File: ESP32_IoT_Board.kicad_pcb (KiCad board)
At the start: 4 copper layers, 127.9 x 63.9 mm, 98 parts, among them J1 SS-52400-002, J2 B2B-PH-SM4-TB, J3 GSD090012SEU, J4 Conn_01x04_Pin, Q1 TEMT6000X01, Q2 BC817, Q3 BC817, U1 MCP73871-2CAI_ML, U2 BME280, U3 ESP32-C3-WROOM-02-H4, U4 CP2102N-Axx-xQFN20, U5 USBLC6-2SC6, U6 W25Q32JVSSIQ, U7 MAX4466EXK, U8 LM1117MPX-3.3

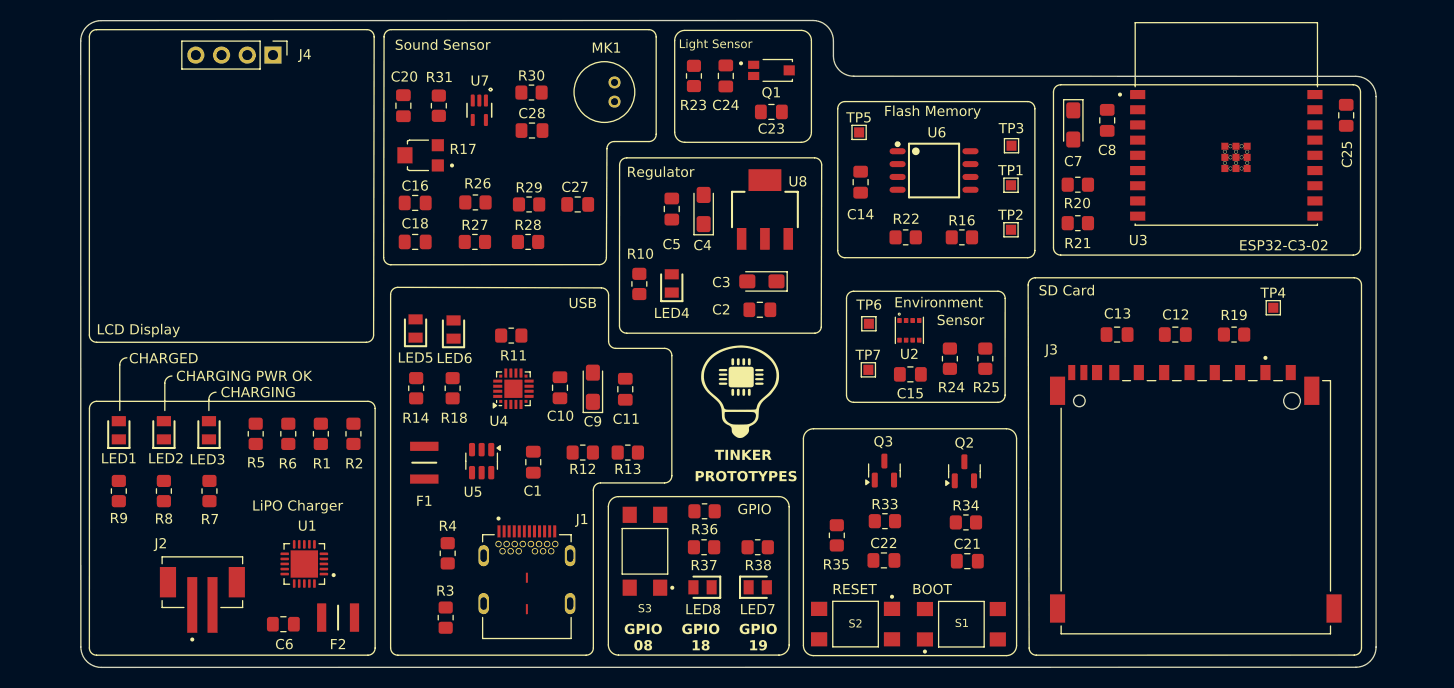
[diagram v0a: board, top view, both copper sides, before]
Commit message: route completed
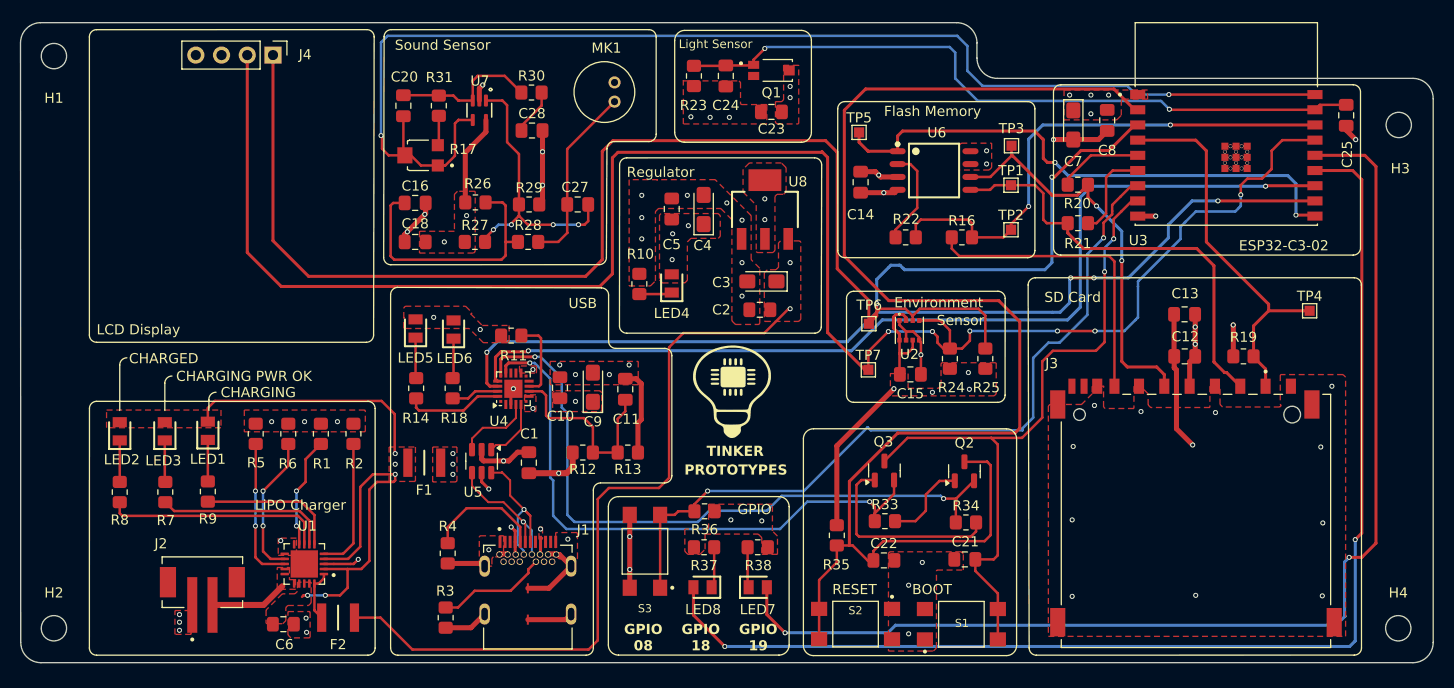
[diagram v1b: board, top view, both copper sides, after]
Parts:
- added H1: MountingHole, MountingHole:MountingHole_2.5mm, F.Cu at (24.8, 30.9)
- added H2: MountingHole, MountingHole:MountingHole_2.5mm, F.Cu at (24.8, 87.3)
- added H3: MountingHole, MountingHole:MountingHole_2.5mm, F.Cu at (157.6, 37.6)
- added H4: MountingHole, MountingHole:MountingHole_2.5mm, F.Cu at (157.6, 87.3)
- moved LED1 8.79 mm to (40.0, 67.8)
- moved R9 8.79 mm to (40.0, 73.8)
- moved C13 6.96 mm to (136.4, 56.4)
- moved LED3 4.36 mm to (35.8, 67.9)
- moved R7 4.36 mm to (35.8, 73.9)
- moved LED2 4.36 mm to (31.3, 67.9)
- moved R8 4.36 mm to (31.3, 73.9)
- moved TP4 3.60 mm to (148.8, 56.0)
- moved C12 2.34 mm to (136.5, 60.5)
- moved R19 2.34 mm to (142.3, 60.5)
- moved J3 1.35 mm to (137.6, 76.8)
- moved J1 1.04 mm to (71.6, 86.0)
- moved G*** 0.80 mm to (91.8, 64.0)
- moved C1 0.44 mm to (71.7, 71.0), turned to 90 degrees
- moved C21 0.30 mm to (114.8, 80.5), turned to 180 degrees
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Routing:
- net /ESP32-C3-02/SCL: track 0.00 -> 180.6 mm, vias 0 -> 6
- net /ESP32-C3-02/SDA: track 0.00 -> 165.0 mm, vias 0 -> 2
- net /ESP32-C3-02/EN: track 0.00 -> 138.0 mm
- net /ESP32-C3-02/MIC_OUT: track 0.00 -> 124.2 mm, vias 0 -> 2
- net /ESP32-C3-02/GPIO18: track 0.00 -> 120.4 mm, vias 0 -> 2
- net /ESP32-C3-02/GPIO19: track 0.00 -> 114.1 mm, vias 0 -> 2
- net /ESP32-C3-02/RX_TX: track 0.00 -> 96.8 mm, vias 0 -> 2
- net /ESP32-C3-02/TX_RX: track 0.00 -> 94.3 mm, vias 0 -> 4
- net GND: track 0.00 -> 89.4 mm, vias 0 -> 57
- net /ESP32-C3-02/GPIO08: track 0.00 -> 77.0 mm, vias 0 -> 2
- net /+5V: track 0.00 -> 74.0 mm, vias 0 -> 2
- net /ESP32-C3-02/PHOTO_C: track 0.00 -> 69.7 mm, vias 0 -> 2
- net /ESP32-C3-02/BOOT: track 0.00 -> 68.6 mm, vias 0 -> 2
- net /ESP32-C3-02/RTS: track 0.00 -> 67.2 mm, vias 0 -> 2
- net /+5V_USB: track 0.00 -> 60.6 mm, vias 0 -> 5
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- added copper zone on F.Cu, net +3.3V
- added copper zone on In1.Cu, net +3.3V
- added copper zone on F.Cu, net /+5V
- added copper zone on F.Cu, net /+5V_USB
- added copper zone on In1.Cu, net /+5V_USB
- added copper zone on F.Cu, net /VBAT
- added copper zone on F.Cu, net /VBUS
- added copper zone on In1.Cu, net /VBUS
- added copper zone on F.Cu, net GND
- added copper zone on In2.Cu, net GND
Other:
- board size 127.9 x 63.9 mm -> 139.5 x 63.2 mm
